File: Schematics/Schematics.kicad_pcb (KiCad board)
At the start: 2 copper layers, 85 x 90 mm, 20 parts, among them U1 TP4056, U2 BH1750, U3 BME688, U4 BU30TD3WG, U5 NRF52840-DONGLE, U6 LIS3DH

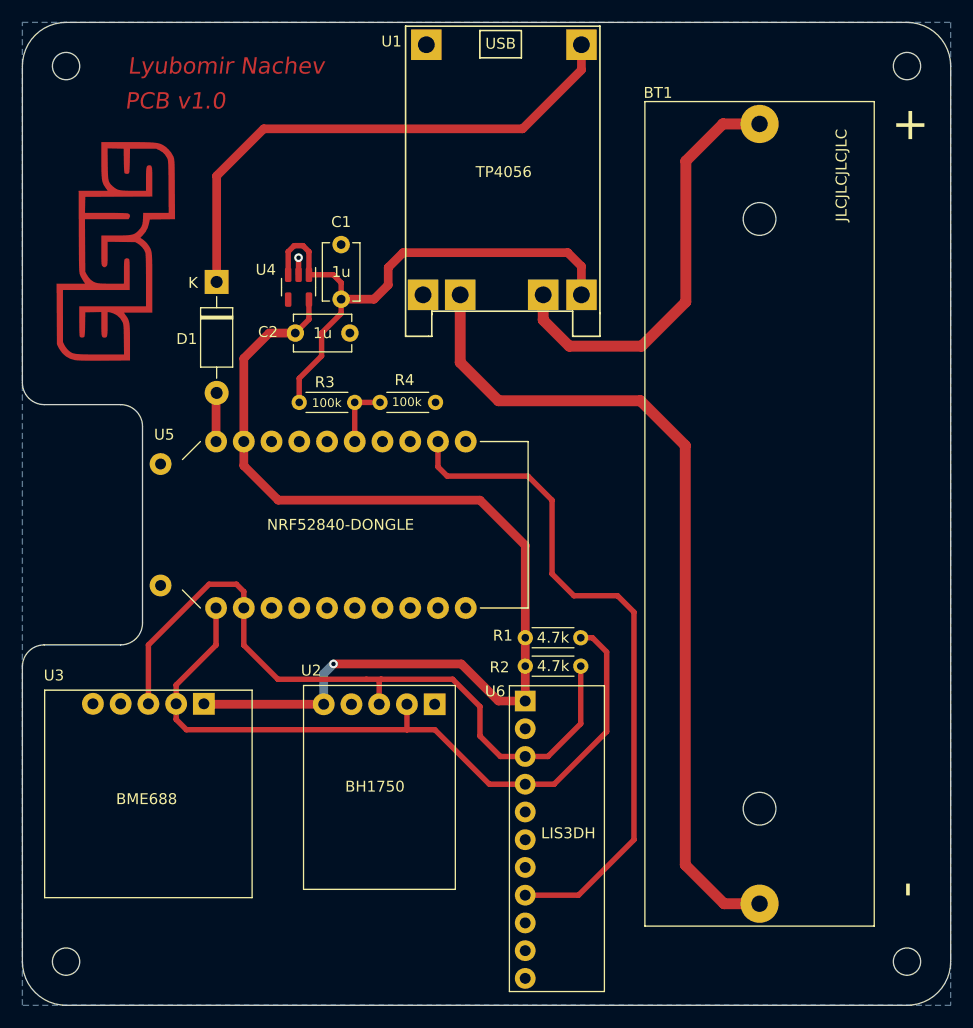
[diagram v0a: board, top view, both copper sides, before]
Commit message: Final commit
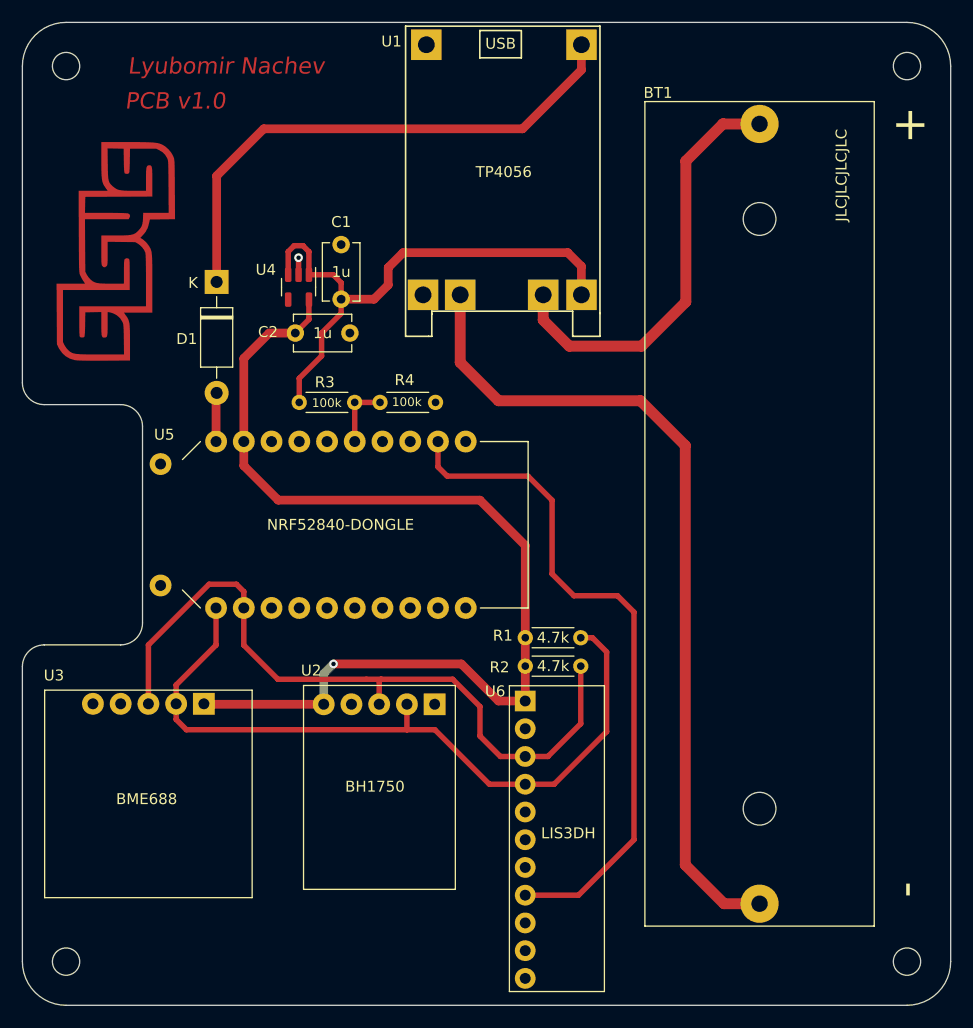
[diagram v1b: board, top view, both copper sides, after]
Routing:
- removed copper zone on B.Cu, net GNDD
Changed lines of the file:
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@@
   (segment (start 156.598 94.646) (end 160.698 98.746) (width 1) (layer "F.Cu") (net 33))
   (segment (start 143.598 94.646) (end 156.598 94.646) (width 1) (layer "F.Cu") (net 33))
-  (zone (net 2) (net_name "GNDD") (layer "B.Cu") (hatch edge 0.508)
-    (connect_pads (clearance 0.3))
-    (min_thickness 0.2) (filled_areas_thickness no)
-    (fill yes (thermal_gap 0.5) (thermal_bridge_width 0.5))
-    (polygon
-      (pts
-        (xy 185 150)
-        (xy 100 150)
-        (xy 100 60)
-        (xy 185 60)
-      )
-    )
-  )
 )
